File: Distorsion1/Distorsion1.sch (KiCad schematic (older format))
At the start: 38 parts, among them J1 Jack-DC, J2 IN, J3 OUT, Sw1 Footswitch, U1 TL082

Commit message: Update 1.1- cambio de isteresis y buffer (esquematico)
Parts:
- removed C2: 2.2uF, Capacitor_SMD:C_0805_2012Metric_Pad1.15x1.40mm_HandSolder, symbol Device:C_Small
- removed C4: 2.2uF, Capacitor_THT:C_Radial_D5.0mm_H5.0mm_P2.00mm, symbol Device:CP1_Small
- removed C5: 4.7uF, Capacitor_THT:C_Radial_D5.0mm_H5.0mm_P2.00mm, symbol Device:CP1_Small
- removed C6: 4.7uF, Capacitor_SMD:C_0805_2012Metric_Pad1.15x1.40mm_HandSolder, symbol Device:C_Small
- removed R11: 1K, Resistor_SMD:R_0805_2012Metric_Pad1.15x1.40mm_HandSolder, symbol Device:R
- removed R6: 47R, Resistor_SMD:R_0805_2012Metric_Pad1.15x1.40mm_HandSolder, symbol Device:R
- added C4: 100nF, Capacitor_SMD:C_0805_2012Metric_Pad1.18x1.45mm_HandSolder, symbol Device:C_Small
- added R4: 1K, Resistor_SMD:R_0805_2012Metric_Pad1.20x1.40mm_HandSolder, symbol Device:R
- added RV1: 10K, Connector_PinSocket_2.54mm:PinSocket_1x03_P2.54mm_Vertical, symbol Device:R_POT
- added unit 2 of U1
- C1: footprint Capacitor_Tantalum_SMD:CP_EIA-7343-30_AVX-N_Pad2.25x2.55mm_HandSolder -> Capacitor_SMD:C_0805_2012Metric_Pad1.18x1.45mm_HandSolder
- C2: renamed from C3; footprint Capacitor_SMD:C_0805_2012Metric_Pad1.15x1.40mm_HandSolder -> Capacitor_SMD:C_0805_2012Metric_Pad1.18x1.45mm_HandSolder
- C3: renamed from C7; footprint Capacitor_SMD:C_0805_2012Metric_Pad1.15x1.40mm_HandSolder -> Capacitor_SMD:C_0805_2012Metric_Pad1.18x1.45mm_HandSolder
- C5: renamed from C8; footprint Capacitor_SMD:C_0805_2012Metric_Pad1.15x1.40mm_HandSolder -> Capacitor_SMD:C_0805_2012Metric_Pad1.18x1.45mm_HandSolder
- C7: renamed from C10; footprint Capacitor_SMD:C_0805_2012Metric_Pad1.15x1.40mm_HandSolder -> Capacitor_SMD:C_0805_2012Metric_Pad1.18x1.45mm_HandSolder
- C8: renamed from C11; footprint Capacitor_SMD:C_0805_2012Metric_Pad1.15x1.40mm_HandSolder -> Capacitor_SMD:C_0805_2012Metric_Pad1.18x1.45mm_HandSolder
- C9: renamed from C12; footprint Capacitor_SMD:C_0805_2012Metric_Pad1.15x1.40mm_HandSolder -> Capacitor_SMD:C_0805_2012Metric_Pad1.18x1.45mm_HandSolder
- R1, R2, R3: footprint Resistor_SMD:R_0805_2012Metric_Pad1.15x1.40mm_HandSolder -> Resistor_SMD:R_0805_2012Metric_Pad1.20x1.40mm_HandSolder
- R10: renamed from R8; footprint Resistor_SMD:R_0805_2012Metric_Pad1.15x1.40mm_HandSolder -> Resistor_SMD:R_0805_2012Metric_Pad1.20x1.40mm_HandSolder
- R11: renamed from R12; footprint Resistor_SMD:R_0805_2012Metric_Pad1.15x1.40mm_HandSolder -> Resistor_SMD:R_0805_2012Metric_Pad1.20x1.40mm_HandSolder
- R5: renamed from R9; footprint Resistor_SMD:R_0805_2012Metric_Pad1.15x1.40mm_HandSolder -> Resistor_SMD:R_0805_2012Metric_Pad1.20x1.40mm_HandSolder
- R6: renamed from R10; footprint Resistor_SMD:R_0805_2012Metric_Pad1.15x1.40mm_HandSolder -> Resistor_SMD:R_0805_2012Metric_Pad1.20x1.40mm_HandSolder
- R7: value 560R -> 1K; footprint Resistor_SMD:R_0805_2012Metric_Pad1.15x1.40mm_HandSolder -> Resistor_SMD:R_0805_2012Metric_Pad1.20x1.40mm_HandSolder
- R8: renamed from R4; footprint Resistor_SMD:R_0805_2012Metric_Pad1.15x1.40mm_HandSolder -> Resistor_SMD:R_0805_2012Metric_Pad1.20x1.40mm_HandSolder
- R9: renamed from R5; footprint Resistor_SMD:R_0805_2012Metric_Pad1.15x1.40mm_HandSolder -> Resistor_SMD:R_0805_2012Metric_Pad1.20x1.40mm_HandSolder
- Sw1: symbol SamacSys_Parts:Footswitch -> Distorsion1-rescue:Footswitch-SamacSys_Parts
- renumbered C9 to C6, RV1 to RV2, RV2 to RV3, RV3 to RV5
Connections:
- wire segments 116 -> 119
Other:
- moved on the sheet: C1, C2, C3, C5, C6, C7, C8, C9, D1, D2, D3, D4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

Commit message: Add local library
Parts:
- C1, C6: symbol Device:CP1_Small -> Distorsion1-rescue:CP1_Small-Device
- C2, C3, C4, C5, C7, C8, C9: symbol Device:C_Small -> Distorsion1-rescue:C_Small-Device
- D1, D2, D4, D5: symbol Device:D_Small -> Distorsion1-rescue:D_Small-Device
- D3, D6: symbol Device:LED -> Distorsion1-rescue:LED-Device
- J1: symbol Connector:Jack-DC -> Distorsion1-rescue:Jack-DC-Connector
- J2, J3: footprint SamacSys_Parts:NYS2162U -> Distorsion1:NYS2162U; symbol Connector:Barrel_Jack_MountingPin -> Distorsion1-rescue:Barrel_Jack_MountingPin-Connector
- R1, R10, R11, R2, R3, R4, R5, R6, R7, R8, R9: symbol Device:R -> Distorsion1-rescue:R-Device
- RV1, RV2, RV3, RV5: symbol Device:R_POT -> Distorsion1-rescue:R_POT-Device
- U1: symbol Amplifier_Operational:TL082 -> Distorsion1-rescue:TL082-Amplifier_Operational
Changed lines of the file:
@@
 $EndDescr
 $Comp
-L Amplifier_Operational:TL082 U1
+L Distorsion1-rescue:TL082-Amplifier_Operational U1
 U 3 1 5ED7479B
 P 2530 1340
@@
 $EndComp
 $Comp
-L Connector:Jack-DC J1
+L Distorsion1-rescue:Jack-DC-Connector J1
 U 1 1 5ED8289C
 P 1160 1355
@@
 $EndComp
 $Comp
-L power:+12V #PWR01
+L Distorsion1-rescue:+12V-power #PWR01
 U 1 1 5ED8C369
 P 1745 1090
@@
 	1745 1255 1745 1090
 $Comp
-L power:GND #PWR02
+L Distorsion1-rescue:GND-power #PWR02
 U 1 1 5ED8DA6B
 P 1745 1630
@@
 	2430 965  2430 1040
 $Comp
-L Device:R R8
+L Distorsion1-rescue:R-Device R8
 U 1 1 5ED98E74
 P 3175 1180
@@
 $EndComp
 $Comp
-L Device:R R9
+L Distorsion1-rescue:R-Device R9
 U 1 1 5ED994B2
 P 3175 1565
@@
 	3175 1330 3175 1375
 $Comp
-L power:GND #PWR09
+L Distorsion1-rescue:GND-power #PWR09
 U 1 1 5ED8E931
 P 2430 1715
@@
 $EndComp
 $Comp
-L power:GND #PWR015
+L Distorsion1-rescue:GND-power #PWR015
 U 1 1 5ED9C0B7
 P 3175 1775
@@
 	3175 1775 3175 1715
 $Comp
-L power:+12V #PWR08
+L Distorsion1-rescue:+12V-power #PWR08
 U 1 1 5ED9350A
 P 2430 965
@@
 $EndComp
 $Comp
-L power:+12V #PWR014
+L Distorsion1-rescue:+12V-power #PWR014
 U 1 1 5ED9D85B
 P 3175 970
@@
 	3175 1375 3175 1415
 $Comp
-L power:+6V #PWR017
+L Distorsion1-rescue:+6V-power #PWR017
 U 1 1 5EDA13BF
 P 3540 975
@@
 $EndComp
 $Comp
-L Device:CP1_Small C1
+L Distorsion1-rescue:CP1_Small-Device C1
 U 1 1 5EDCFD93
 P 2075 1350
@@
 $EndComp
 $Comp
-L power:+12V #PWR04
+L Distorsion1-rescue:+12V-power #PWR04
 U 1 1 5EDD0D8D
 P 2075 1030
@@
 	2075 1030 2075 1250
 $Comp
-L power:GND #PWR05
+L Distorsion1-rescue:GND-power #PWR05
 U 1 1 5EDD3194
 P 2075 1725
@@
 	2075 1725 2075 1450
 $Comp
-L Device:LED D3
+L Distorsion1-rescue:LED-Device D3
 U 1 1 5EEDE03A
 P 4200 1160
@@
 $EndComp
 $Comp
-L Device:R R10
+L Distorsion1-rescue:R-Device R10
 U 1 1 5EEE103C
 P 4200 1510
@@
 	4200 1310 4200 1360
 $Comp
-L power:GND #PWR019
+L Distorsion1-rescue:GND-power #PWR019
 U 1 1 5EEE43E8
 P 4200 1775
@@
 	4200 1775 4200 1660
 $Comp
-L power:+12V #PWR018
+L Distorsion1-rescue:+12V-power #PWR018
 U 1 1 5EEE7291
 P 4200 955
@@
 	4200 955  4200 1010
 $Comp
-L Device:LED D6
+L Distorsion1-rescue:LED-Device D6
 U 1 1 5EDE8659
 P 4845 1140
@@
 $EndComp
 $Comp
-L Device:R R11
+L Distorsion1-rescue:R-Device R11
 U 1 1 5EDE8663
 P 5750 1455
@@
 $EndComp
 $Comp
-L power:GND #PWR0101
+L Distorsion1-rescue:GND-power #PWR0101
 U 1 1 5EDE866E
 P 5750 1720
@@
 	5750 1720 5750 1605
 $Comp
-L power:+12V #PWR0102
+L Distorsion1-rescue:+12V-power #PWR0102
 U 1 1 5EDE8679
 P 4595 950
@@
 	5750 1190 5605 1190
 $Comp
-L Connector:Barrel_Jack_MountingPin J3
+L Distorsion1-rescue:Barrel_Jack_MountingPin-Connector J3
 U 1 1 5EE03F35
 P 9960 3990
 F 0 "J3" H 9730 3954 50  0000 R CNN
 F 1 "OUT" H 9730 3863 50  0000 R CNN
-F 2 "SamacSys_Parts:NYS2162U" H 10010 3950 50  0001 C CNN
+F 2 "Distorsion1:NYS2162U" H 10010 3950 50  0001 C CNN
 F 3 "~" H 10010 3950 50  0001 C CNN
 F 4 "NYS2162-U" H 9960 3990 50  0001 C CNN "manf#"
@@
 $EndComp
 $Comp
-L power:GND #PWR024
+L Distorsion1-rescue:GND-power #PWR024
 U 1 1 5EE07C66
 P 9515 4225
@@
 	9515 4090 9660 4090
 $Comp
-L Device:R R5
+L Distorsion1-rescue:R-Device R5
 U 1 1 5EE19AE5
 P 6090 3195
@@
 $EndComp
 $Comp
-L Device:C_Small C8
+L Distorsion1-rescue:C_Small-Device C8
 U 1 1 5EE1A1D6
 P 6075 3740
@@
 $EndComp
 $Comp
-L Device:R R6
+L Distorsion1-rescue:R-Device R6
 U 1 1 5EE1A9C1
 P 6420 3930
@@
 $EndComp
 $Comp
-L Device:R_POT RV3
+L Distorsion1-rescue:R_POT-Device RV3
 U 1 1 5EE1AFD0
 P 6420 3470
@@
 $EndComp
 $Comp
-L Device:C_Small C9
+L Distorsion1-rescue:C_Small-Device C9
 U 1 1 5EE26A33
 P 6420 3030
@@
 $EndComp
 $Comp
-L power:GND #PWR021
+L Distorsion1-rescue:GND-power #PWR021
 U 1 1 5EE270F4
 P 6215 2815
@@
 Connection ~ 6420 3740
 $Comp
-L power:GND #PWR022
+L Distorsion1-rescue:GND-power #PWR022
 U 1 1 5EE3147C
 P 6420 4140
@@
 Tone Control
 $Comp
-L Device:R_POT RV5
+L Distorsion1-rescue:R_POT-Device RV5
 U 1 1 5EDE9830
 P 8270 3840
@@
 $EndComp
 $Comp
-L power:GND #PWR023
+L Distorsion1-rescue:GND-power #PWR023
 U 1 1 5EDFD2FF
 P 8270 4160
@@
 	3325 4925 3325 5030
 $Comp
-L power:GND #PWR0103
+L Distorsion1-rescue:GND-power #PWR0103
 U 1 1 5FC74459
 P 3325 5030
@@
 	3325 4725 3325 4670
 $Comp
-L Device:C_Small C4
+L Distorsion1-rescue:C_Small-Device C4
 U 1 1 5FC6C037
 P 3325 4825
@@
 	3890 4060 3890 4215
 $Comp
-L Device:R_POT RV1
+L Distorsion1-rescue:R_POT-Device RV1
 U 1 1 5FBE46EF
 P 3325 4435
@@
 $EndComp
 $Comp
-L Device:R R4
+L Distorsion1-rescue:R-Device R4
 U 1 1 5FC32941
 P 3580 4215
@@
 $EndComp
 $Comp
-L Device:R R3
+L Distorsion1-rescue:R-Device R3
 U 1 1 5ED95416
 P 3245 3355
@@
 	2300 3845 2300 3780
 $Comp
-L power:GND #PWR06
+L Distorsion1-rescue:GND-power #PWR06
 U 1 1 5EDB4AA6
 P 2300 3845
@@
 	2300 3480 2300 3355
 $Comp
-L Device:R R1
+L Distorsion1-rescue:R-Device R1
 U 1 1 5EDB0F98
 P 2300 3630
@@
 	4340 4060 4695 4060
 $Comp
-L Device:C_Small C5
+L Distorsion1-rescue:C_Small-Device C5
 U 1 1 5EE4162A
 P 4240 4060
@@
 	3555 3760 3555 3665
 $Comp
-L power:GND #PWR016
+L Distorsion1-rescue:GND-power #PWR016
 U 1 1 5EE2C41A
 P 3555 3760
@@
 	4240 3735 4240 3655
 $Comp
-L Device:R_POT RV2
+L Distorsion1-rescue:R_POT-Device RV2
 U 1 1 5EDE8583
 P 4240 3885
@@
 	3555 3465 3555 3355
 $Comp
-L Device:C_Small C3
+L Distorsion1-rescue:C_Small-Device C3
 U 1 1 5EDDBD2F
 P 3555 3565
@@
 $EndComp
 $Comp
-L Device:C_Small C2
+L Distorsion1-rescue:C_Small-Device C2
 U 1 1 5ED89C24
 P 2520 3355
@@
 $EndComp
 $Comp
-L Device:R R2
+L Distorsion1-rescue:R-Device R2
 U 1 1 5EDA2255
 P 2985 3065
@@
 $EndComp
 $Comp
-L power:+6V #PWR011
+L Distorsion1-rescue:+6V-power #PWR011
 U 1 1 5EDA7A9C
 P 2985 2825
@@
 	4845 3215 4695 3215
 $Comp
-L Device:C_Small C7
+L Distorsion1-rescue:C_Small-Device C7
 U 1 1 5EEA0806
 P 4945 3215
@@
 	1985 3660 1985 3505
 $Comp
-L power:GND #PWR03
+L Distorsion1-rescue:GND-power #PWR03
 U 1 1 5EE01F05
 P 1985 3660
@@
 $EndComp
 $Comp
-L power:GND #PWR020
+L Distorsion1-rescue:GND-power #PWR020
 U 1 1 5EDDE0D5
 P 5345 3980
@@
 	5395 3635 5395 3455
 $Comp
-L Device:D_Small D5
+L Distorsion1-rescue:D_Small-Device D5
 U 1 1 5EDD7029
 P 5395 3735
@@
 $EndComp
 $Comp
-L Device:D_Small D4
+L Distorsion1-rescue:D_Small-Device D4
 U 1 1 5EDD701F
 P 5290 3740
@@
 	4140 4380 3890 4380
 $Comp
-L Device:D_Small D2
+L Distorsion1-rescue:D_Small-Device D2
 U 1 1 5EDC43EE
 P 4245 4490
@@
 	4090 3885 3890 3885
 $Comp
-L Device:D_Small D1
+L Distorsion1-rescue:D_Small-Device D1
 U 1 1 5EDB2C53
 P 4240 4380
@@
 $EndComp
 $Comp
-L Device:CP1_Small C6
+L Distorsion1-rescue:CP1_Small-Device C6
 U 1 1 5ED8BDA6
 P 4940 3455
@@
 $EndComp
 $Comp
-L Connector:Barrel_Jack_MountingPin J2
+L Distorsion1-rescue:Barrel_Jack_MountingPin-Connector J2
 U 1 1 5ED87E3F
 P 740 3405
 F 0 "J2" H 797 3722 50  0000 C CNN
 F 1 "IN" H 797 3631 50  0000 C CNN
-F 2 "SamacSys_Parts:NYS2162U" H 790 3365 50  0001 C CNN
+F 2 "Distorsion1:NYS2162U" H 790 3365 50  0001 C CNN
 F 3 "~" H 790 3365 50  0001 C CNN
 F 4 "NYS2162-U" H 740 3405 50  0001 C CNN "manf#"
@@
 $EndComp
 $Comp
-L Amplifier_Operational:TL082 U1
+L Distorsion1-rescue:TL082-Amplifier_Operational U1
 U 1 1 5ED754E2
 P 4280 3455
@@
 Connection ~ 5395 3455
 $Comp
-L Amplifier_Operational:TL082 U1
+L Distorsion1-rescue:TL082-Amplifier_Operational U1
 U 2 1 5FBFF2A8
 P 7520 3565
@@
 	5775 3455 5775 3740
 $Comp
-L Device:R R7
+L Distorsion1-rescue:R-Device R7
 U 1 1 5FB9D050
 P 6780 3470

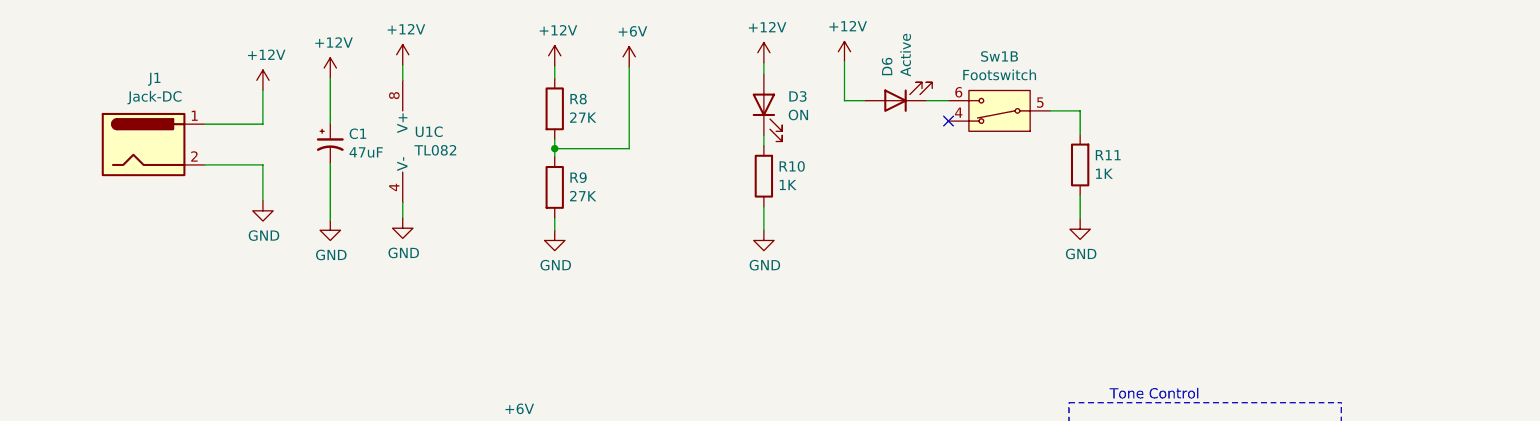
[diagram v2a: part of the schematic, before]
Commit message: PCB 1.0
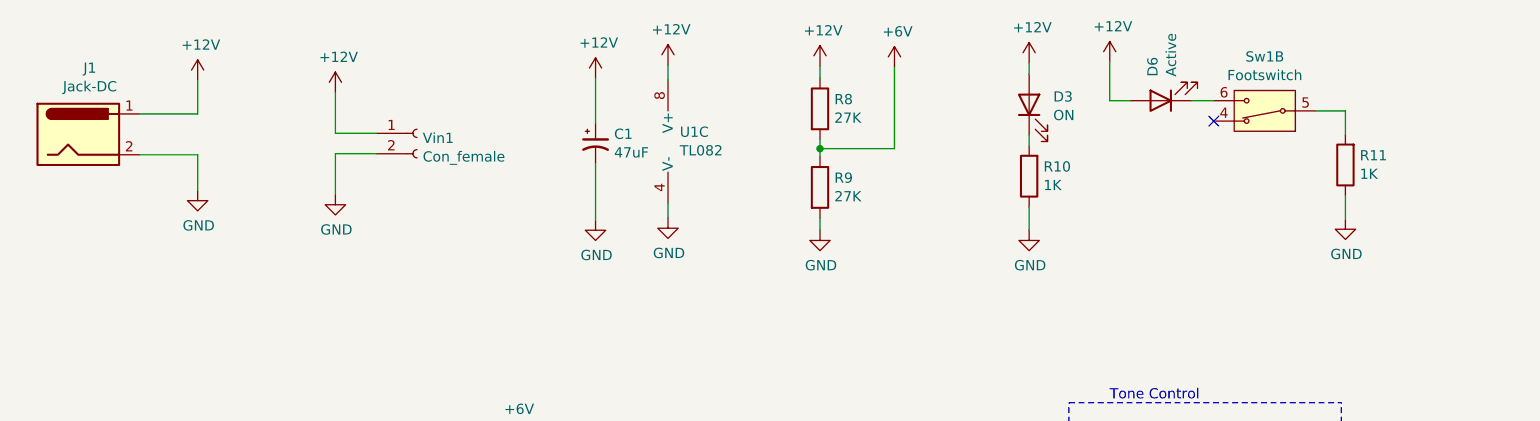
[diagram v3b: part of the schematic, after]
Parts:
- added Vin1: Con_female, Connector_PinHeader_2.54mm:PinHeader_1x02_P2.54mm_Vertical, symbol Connector:Conn_01x02_Female
- Sw1: footprint SamacSys_Parts:FS57003PLT2B2M2QE -> Distorsion1:FS57003PLT2B2M2QE
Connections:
- net +12V: now also Vin1.1 (Pin_1)
- net GND: now also Vin1.2 (Pin_2)
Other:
- moved on the sheet: C1, D3, D6, J1, R10, R11, R8, R9, Sw1B, U1C
